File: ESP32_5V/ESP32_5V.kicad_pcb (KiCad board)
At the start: 4 copper layers, 90 x 60 mm, 48 parts, among them J10 Conn_01x11, J11 Conn_01x11, J12 Conn_01x11, J13 Conn_01x11, J15 Screw_Terminal_01x11, J16 Screw_Terminal_01x11, J17 Barrel_Jack_MountingPin, J2 Conn_01x11, J3 Conn_01x11, J4 Conn_01x11, J5 Conn_01x11, J6 Conn_01x11, J7 Conn_01x11, J8 Conn_01x11, J9 Conn_01x11, U1 SN74LVC245APW, U2 SN74LVC245APW, U4 TPS563201, U5 SN74LVC245APW

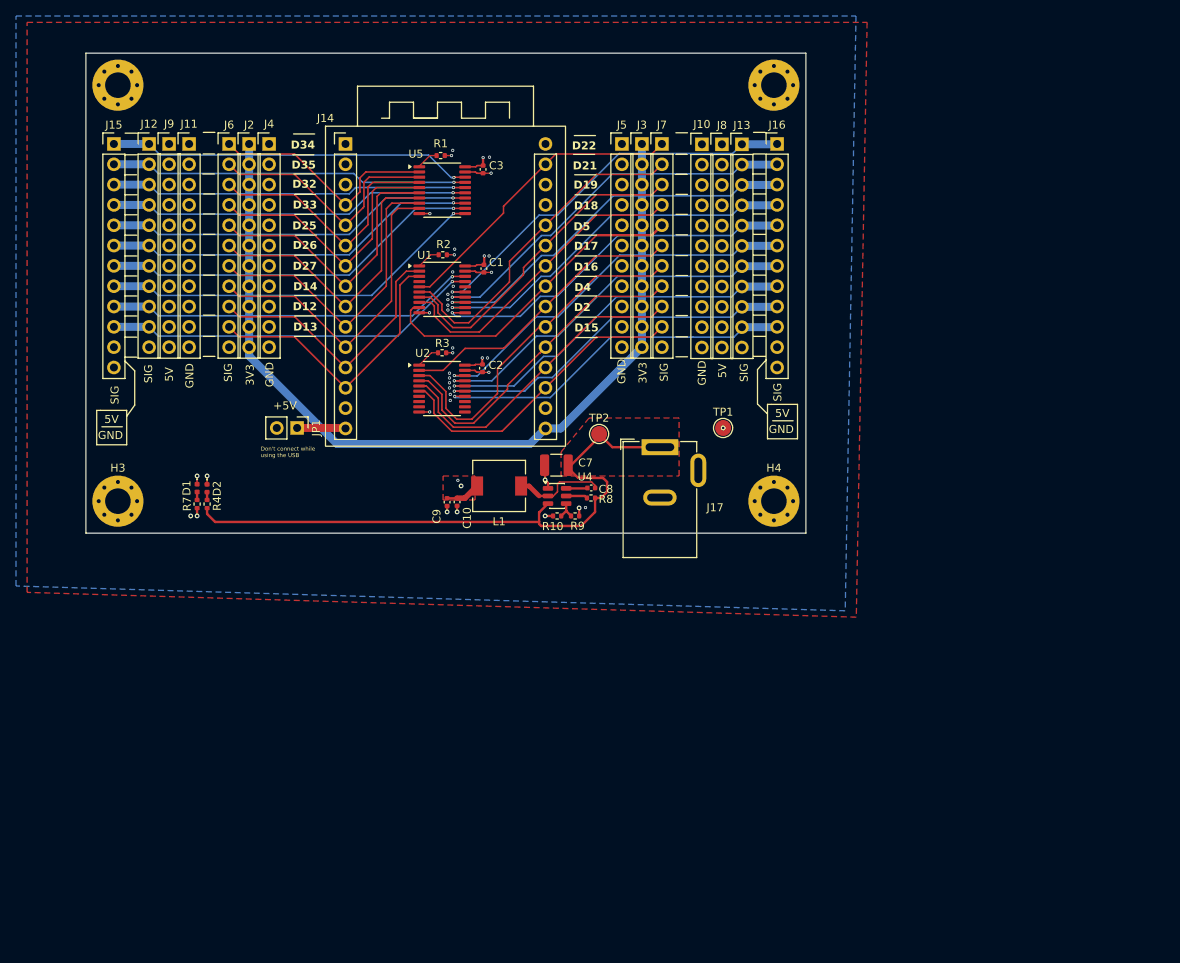
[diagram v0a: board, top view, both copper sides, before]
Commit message: update
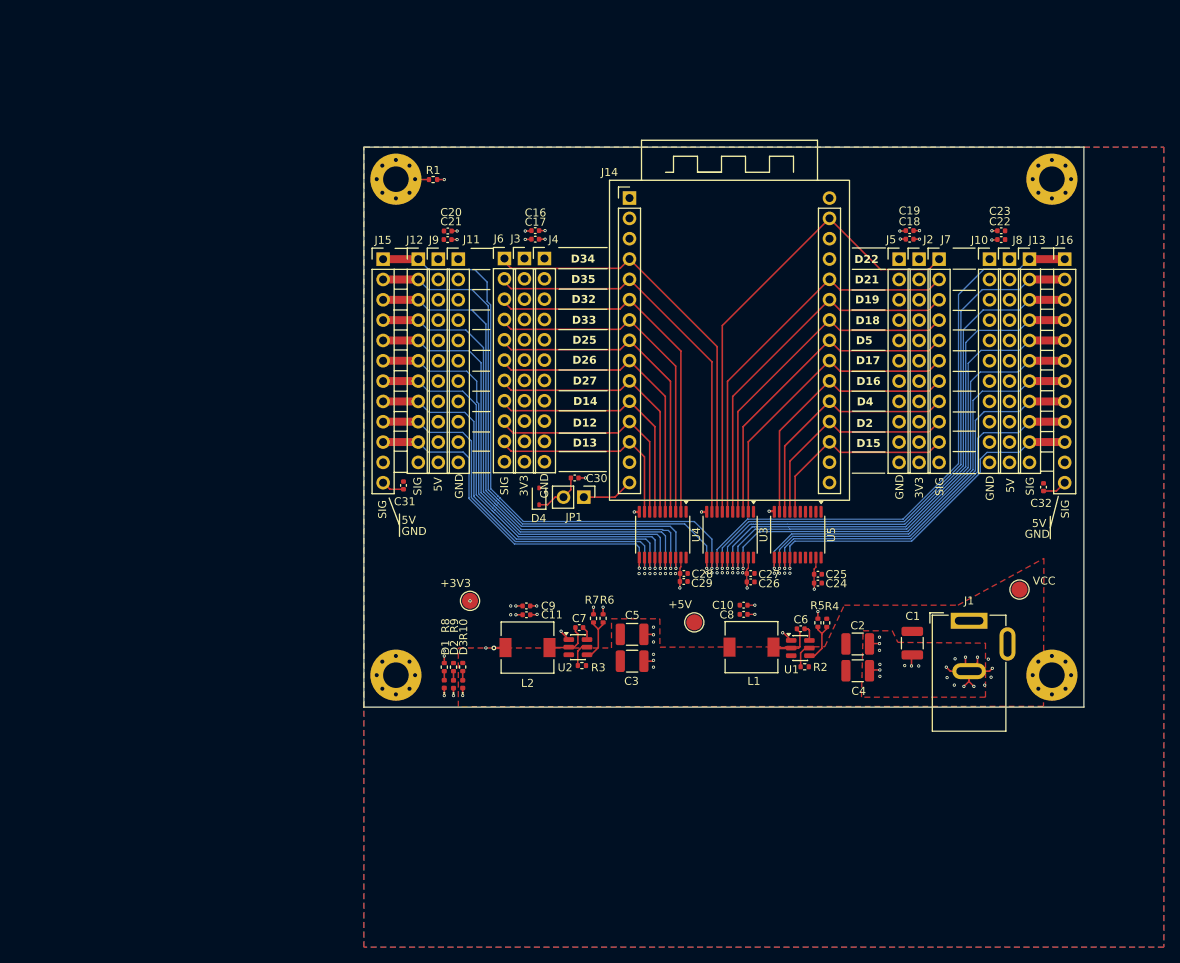
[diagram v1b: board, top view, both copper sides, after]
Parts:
- removed J17: Barrel_Jack_MountingPin, Connector_BarrelJack:BarrelJack_GCT_DCJ200-10-A_Horizontal
- removed the REF** at (104.5, 73.1)
- removed the REF** at (104.0, 62.0)
- removed the REF** at (103.7, 49.1)
- added C11: 10u, Capacitor_SMD:C_0402_1005Metric, F.Cu at (113.9, 101.8)
- added C16: 10u, Capacitor_SMD:C_0402_1005Metric, F.Cu at (115.0, 53.8)
- added C17: 10u, Capacitor_SMD:C_0402_1005Metric, F.Cu at (115.0, 54.9)
- added C18: 10u, Capacitor_SMD:C_0402_1005Metric, F.Cu at (161.8, 54.9)
- added C19: 10u, Capacitor_SMD:C_0402_1005Metric, F.Cu at (161.8, 53.8)
- added C20: 10u, Capacitor_SMD:C_0402_1005Metric, F.Cu at (104.1, 53.9)
- added C21: 10u, Capacitor_SMD:C_0402_1005Metric, F.Cu at (104.1, 55.0)
- added C22: 10u, Capacitor_SMD:C_0402_1005Metric, F.Cu at (173.3, 55.0)
- added C23: 10u, Capacitor_SMD:C_0402_1005Metric, F.Cu at (173.3, 53.9)
- added C24: 100nF, Capacitor_SMD:C_0402_1005Metric, F.Cu at (150.3, 97.9)
- added C25: 100nF, Capacitor_SMD:C_0402_1005Metric, F.Cu at (150.4, 96.8)
- added C26: 100nF, Capacitor_SMD:C_0402_1005Metric, F.Cu at (141.9, 97.7)
- added C27: 100nF, Capacitor_SMD:C_0402_1005Metric, F.Cu at (141.9, 96.7)
- added C28: 100nF, Capacitor_SMD:C_0402_1005Metric, F.Cu at (133.6, 96.7)
- added C29: 100nF, Capacitor_SMD:C_0402_1005Metric, F.Cu at (133.6, 97.7)
- added C30: 10u, Capacitor_SMD:C_0402_1005Metric, F.Cu at (120.0, 84.8)
- added C31: 10u, Capacitor_SMD:C_0402_1005Metric, F.Cu at (98.5, 85.7)
- added C32: 10u, Capacitor_SMD:C_0402_1005Metric, F.Cu at (178.6, 85.9)
- added C4: 10u, Capacitor_SMD:C_1210_3225Metric, F.Cu at (155.3, 108.8)
- added C5: 10u, Capacitor_SMD:C_1210_3225Metric, F.Cu at (127.1, 104.3)
- added C6: 100nF, Capacitor_SMD:C_0402_1005Metric, F.Cu at (148.2, 103.6)
- added D3: LED, LED_SMD:LED_0402_1005Metric, F.Cu at (106.0, 110.5)
- added D4: 1N5819WS, Diode_SMD:D_SOD-323, F.Cu at (115.5, 87.0)
- added J1: Barrel_Jack_MountingPin, Connector_BarrelJack:BarrelJack_GCT_DCJ200-10-A_Horizontal, F.Cu at (169.2, 102.6)
- added L2: 4,7uH, Inductor_SMD:L_6.3x6.3_H3, F.Cu at (114.0, 106.0)
- added R5: 10k, Resistor_SMD:R_0402_1005Metric, F.Cu at (150.3, 102.8)
- added R6: 33k, Resistor_SMD:R_0402_1005Metric, F.Cu at (123.5, 102.3)
- added REF**: KiCad-Logo2_6mm_SilkScreen, Symbol:KiCad-Logo2_6mm_SilkScreen, B.Cu at (139.2, 52.9)
- added REF**: OSHW-Logo_19x20mm_SilkScreen, Symbol:OSHW-Logo_19x20mm_SilkScreen, B.Cu at (139.4, 71.4)
- added REF**: WEEE-Logo_8.4x12mm_SilkScreen, Symbol:WEEE-Logo_8.4x12mm_SilkScreen, B.Cu at (139.2, 93.2)
- added TP3: TestPoint, TestPoint:TestPoint_Pad_D2.0mm, F.Cu at (134.9, 102.8)
- added U3: SN74LVC245APW, Package_SO:TSSOP-20_4.4x6.5mm_P0.65mm, F.Cu at (139.4, 91.8)
- C1: value 10nF -> 10u; footprint Capacitor_SMD:C_0402_1005Metric -> Capacitor_SMD:C_1210_3225Metric
- C2, C3: value 10nF -> 100n; footprint Capacitor_SMD:C_0402_1005Metric -> Capacitor_SMD:C_1210_3225Metric
- C7: value 10u -> 100nF; footprint Capacitor_SMD:C_1210_3225Metric -> Capacitor_SMD:C_0402_1005Metric
- C8: value 100nF -> 10u
- R10: value 20k -> 500
- R2, R3: value 0 -> 10k
- R4: value 10k -> 51k
- R8: value 10k -> 500
- R9: value 110k -> 500
- U1, U2: value SN74LVC245APW -> TPS563201; footprint Package_SO:TSSOP-20_4.4x6.5mm_P0.65mm -> Package_TO_SOT_SMD:SOT-23-6
- U4: value TPS563201 -> SN74LVC245APW; footprint Package_TO_SOT_SMD:SOT-23-6 -> Package_SO:TSSOP-20_4.4x6.5mm_P0.65mm
- moved H3 118.8 mm to (179.6, 109.4)
- moved J2 85.0 mm to (163.0, 57.4)
- moved R4 78.9 mm to (151.4, 102.9), turned to -90 degrees
- moved C1 71.1 mm to (162.2, 105.4)
- moved R2 68.5 mm to (148.7, 108.3)
- moved C3 64.2 mm to (127.1, 107.7), turned to 0 degrees
- moved U1 63.4 mm to (148.2, 106.0)
- moved U5 61.9 mm to (147.8, 91.8), turned to -90 degrees
- moved C2 58.2 mm to (155.3, 105.5), turned to 0 degrees
- moved H4 52.0 mm to (97.6, 109.4)
- moved R7 51.6 mm to (122.3, 102.3)
- moved R3 42.8 mm to (120.8, 108.2)
- moved TP1 42.2 mm to (175.6, 98.7)
- moved D1 39.4 mm to (103.7, 110.5), turned to 90 degrees
- moved D2 39.4 mm to (104.8, 110.5), turned to 90 degrees
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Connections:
- C1 pad 1: +5V -> VCC
- C2 pad 1: +5V -> VCC
- C3 pad 1: +5V -> VCC
- C7 pad 1: VCC -> Net-(U2-VBST)
- C7 pad 2: GND -> Net-(U2-SW)
- C8 pad 1: Net-(U4-VBST) -> +5V
- C8 pad 2: Net-(U4-SW) -> GND
- C9 pad 1: +5V -> +3V3
- H1 pad 1: GND -> Net-(H1-Pad1)
- H2 pad 1: GND -> unconnected-(H2-Pad1)_3
- H3 pad 1: GND -> unconnected-(H3-Pad1)
- H4 pad 1: GND -> unconnected-(H4-Pad1)_5
- J14 pad 30: +3V3 -> unconnected-(J14-Pad30)
- JP1 pad 2: +5V -> Net-(D4-K)
- L1 pad 1: Net-(U4-SW) -> Net-(U1-SW)
- R1 pad 1: Net-(U5-DIR) -> Net-(H1-Pad1)
- R1 pad 2: +5V -> GND
- R10 pad 1: Net-(U4-VFB) -> VCC
- R10 pad 2: GND -> Net-(D3-A)
- R2 pad 1: Net-(U1-DIR) -> Net-(U1-EN)
- R2 pad 2: +5V -> VCC
- R3 pad 1: Net-(U2-DIR) -> Net-(U2-EN)
- R3 pad 2: +5V -> VCC
- R4 pad 1: VCC -> +5V
- R4 pad 2: Net-(D2-A) -> Net-(U1-VFB)
- R7 pad 1: +5V -> Net-(U2-VFB)
- R7 pad 2: Net-(D1-A) -> GND
- R8 pad 1: Net-(U4-EN) -> +3V3
- R8 pad 2: VCC -> Net-(D1-A)
- R9 pad 2: Net-(U4-VFB) -> Net-(D2-A)
- TP1 pad 1: +5V -> VCC
- TP2 pad 1: VCC -> +3V3
- U1 pad 1: Net-(U1-DIR) -> GND
- U1 pad 2: /Conector_3V3/D12 -> Net-(U1-SW)
- U1 pad 3: /Conector_3V3/D13 -> VCC
- U1 pad 4: unconnected-(U1-A3-Pad4) -> Net-(U1-VFB)
- U1 pad 5: /Conector_3V3/D22 -> Net-(U1-EN)
- U1 pad 6: /Conector_3V3/D21 -> Net-(U1-VBST)
- U2 pad 1: Net-(U2-DIR) -> GND
- U2 pad 2: /Conector_3V3/D17 -> Net-(U2-SW)
- U2 pad 3: /Conector_3V3/D16 -> VCC
- U2 pad 4: /Conector_3V3/D4 -> Net-(U2-VFB)
- U2 pad 5: /Conector_3V3/D2 -> Net-(U2-EN)
- U2 pad 6: /Conector_3V3/D15 -> Net-(U2-VBST)
- U4 pad 1: GND -> +5V
- U4 pad 2: Net-(U4-SW) -> /Conector_3V3/D32
- U4 pad 3: VCC -> /Conector_3V3/D33
- U4 pad 4: Net-(U4-VFB) -> /Conector_3V3/D25
- U4 pad 5: Net-(U4-EN) -> /Conector_3V3/D26
- U4 pad 6: Net-(U4-VBST) -> /Conector_3V3/D27
- U5 pad 1: Net-(U5-DIR) -> +5V
- U5 pad 11: /Conector_5V/D14_5V -> /Conector_5V/D16_5V
- U5 pad 12: /Conector_5V/D27_5V -> /Conector_5V/D4_5V
- U5 pad 13: /Conector_5V/D26_5V -> /Conector_5V/D2_5V
- U5 pad 14: /Conector_5V/D25_5V -> /Conector_5V/D15_5V
- U5 pad 15: /Conector_5V/D33_5V -> unconnected-(U5-B4-Pad15)
- U5 pad 16: /Conector_5V/D32_5V -> unconnected-(U5-B3-Pad16)
- U5 pad 17: /Conector_5V/D35_5V -> unconnected-(U5-B2-Pad17)
- U5 pad 18: /Conector_5V/D34_5V -> unconnected-(U5-B1-Pad18)
- U5 pad 2: /Conector_3V3/D34 -> unconnected-(U5-A1-Pad2)
- U5 pad 3: /Conector_3V3/D35 -> unconnected-(U5-A2-Pad3)
- U5 pad 4: /Conector_3V3/D32 -> unconnected-(U5-A3-Pad4)
- U5 pad 5: /Conector_3V3/D33 -> unconnected-(U5-A4-Pad5)
- U5 pad 6: /Conector_3V3/D25 -> /Conector_3V3/D15
- U5 pad 7: /Conector_3V3/D26 -> /Conector_3V3/D2
- U5 pad 8: /Conector_3V3/D27 -> /Conector_3V3/D4
- U5 pad 9: /Conector_3V3/D14 -> /Conector_3V3/D16
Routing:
- net +3V3: track 110.6 -> 8.18 mm, vias 0 -> 10
- net VCC: track 78.0 -> 0.00 mm
- net GND: track 21.0 -> 59.3 mm, vias 33 -> 78
- net /Conector_5V/D34_5V: track 45.7 -> 75.5 mm
- net /Conector_5V/D35_5V: track 44.8 -> 71.9 mm
- net /Conector_5V/D22_5V: track 49.9 -> 74.6 mm
- net /Conector_3V3/D34: track 29.7 -> 53.0 mm
- net /Conector_5V/D21_5V: track 49.1 -> 71.9 mm
- net /Conector_5V/D32_5V: track 44.7 -> 66.7 mm
- net /Conector_3V3/D22: track 38.2 -> 59.1 mm
- net /Conector_5V/D19_5V: track 48.4 -> 68.9 mm
- net /Conector_3V3/D35: track 31.2 -> 50.2 mm
- net +5V: track 18.9 -> 0.00 mm, vias 10 -> 0
- net /Conector_5V/D18_5V: track 47.6 -> 66.4 mm
- net /Conector_5V/D33_5V: track 45.5 -> 63.3 mm
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- added copper zone on B.Cu, net +3V3
- added copper zone on F.Cu, net GND
- removed copper zone on B.Cu, net +5V
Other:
- board size 90 x 60 mm -> 90 x 70 mm
- board text added: "+3V3"
- board text added: "VCC"
- board text removed: "Don't connect while using the USB"
